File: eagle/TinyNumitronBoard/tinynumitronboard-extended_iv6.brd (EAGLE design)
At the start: 100 x 50 mm, 37 parts

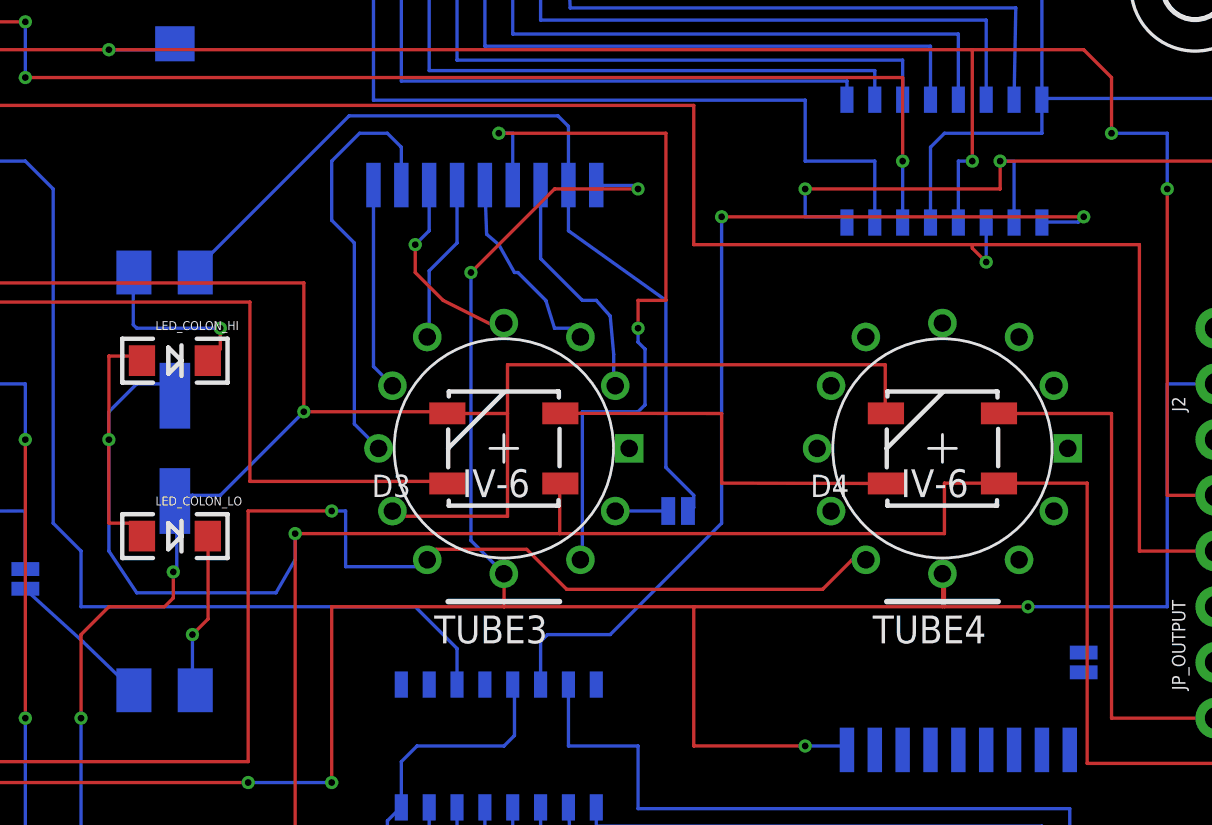
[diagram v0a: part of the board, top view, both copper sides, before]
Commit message: Post 2nd script exec, all look ok
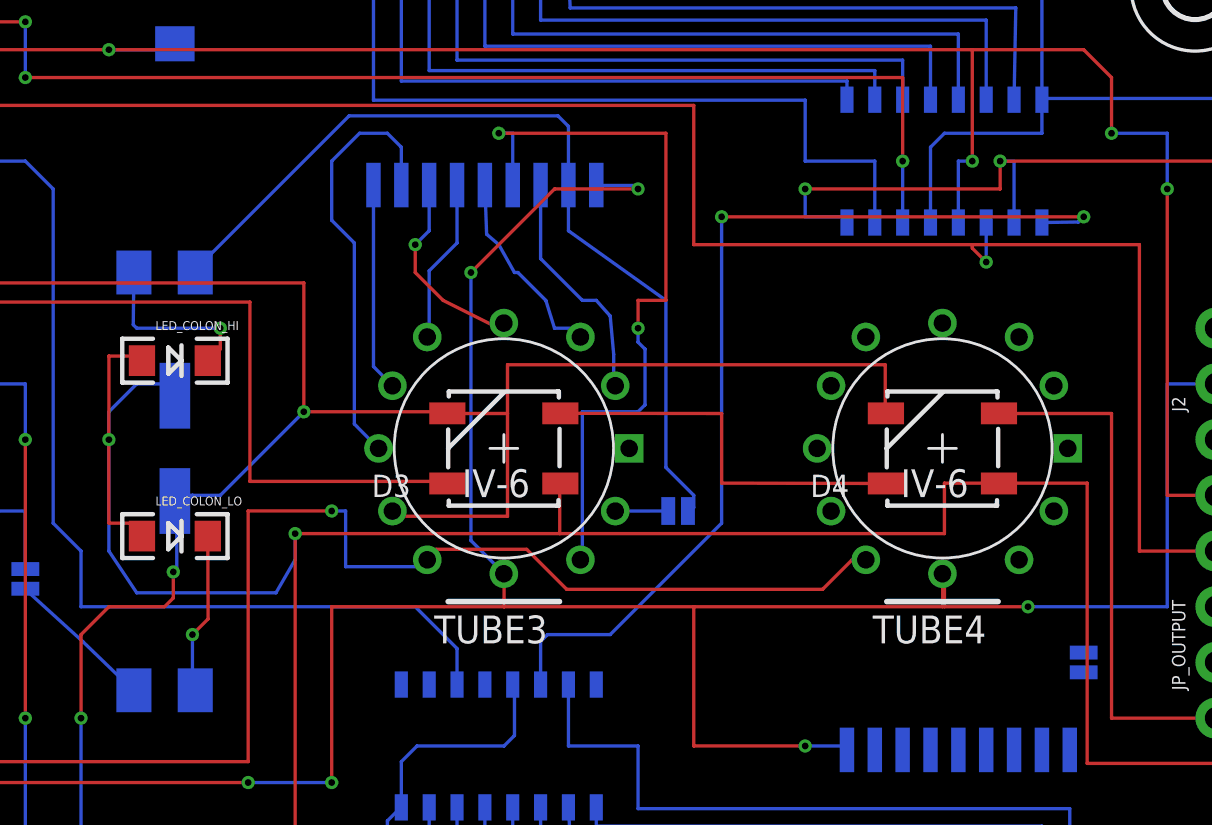
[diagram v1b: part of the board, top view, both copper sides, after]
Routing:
- net N$105: track 45.0 -> 0.00 mm, vias 2 -> 0
- net N$53: track 0.00 -> 44.9 mm, vias 0 -> 2
- net N$99: track 34.2 -> 0.00 mm, vias 2 -> 0
- net N$63: track 0.00 -> 34.2 mm, vias 0 -> 2
- net N$82: track 19.7 -> 0.00 mm
- net N$58: track 0.00 -> 19.7 mm
- net N$64: track 0.00 -> 10.8 mm
- net N$87: track 10.8 -> 0.00 mm
- net N$54: track 0.00 -> 9.51 mm
- net N$81: track 9.49 -> 0.00 mm
- net N$60: track 0.00 -> 9.22 mm, vias 0 -> 1
- net N$84: track 9.20 -> 0.00 mm, vias 1 -> 0
- net N$62: track 0.00 -> 9.07 mm
- net N$86: track 9.05 -> 0.00 mm
- net N$94: track 8.15 -> 0.00 mm, vias 1 -> 0
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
